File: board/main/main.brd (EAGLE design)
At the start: 108.5 x 39 mm, 40 parts, among them IC1 78m05, J1 188275-8, U1 6N138M, U2 MMBD4148TW-7-F, U3 MMBD4148TW-7-F, U4 MMBD4148TW-7-F

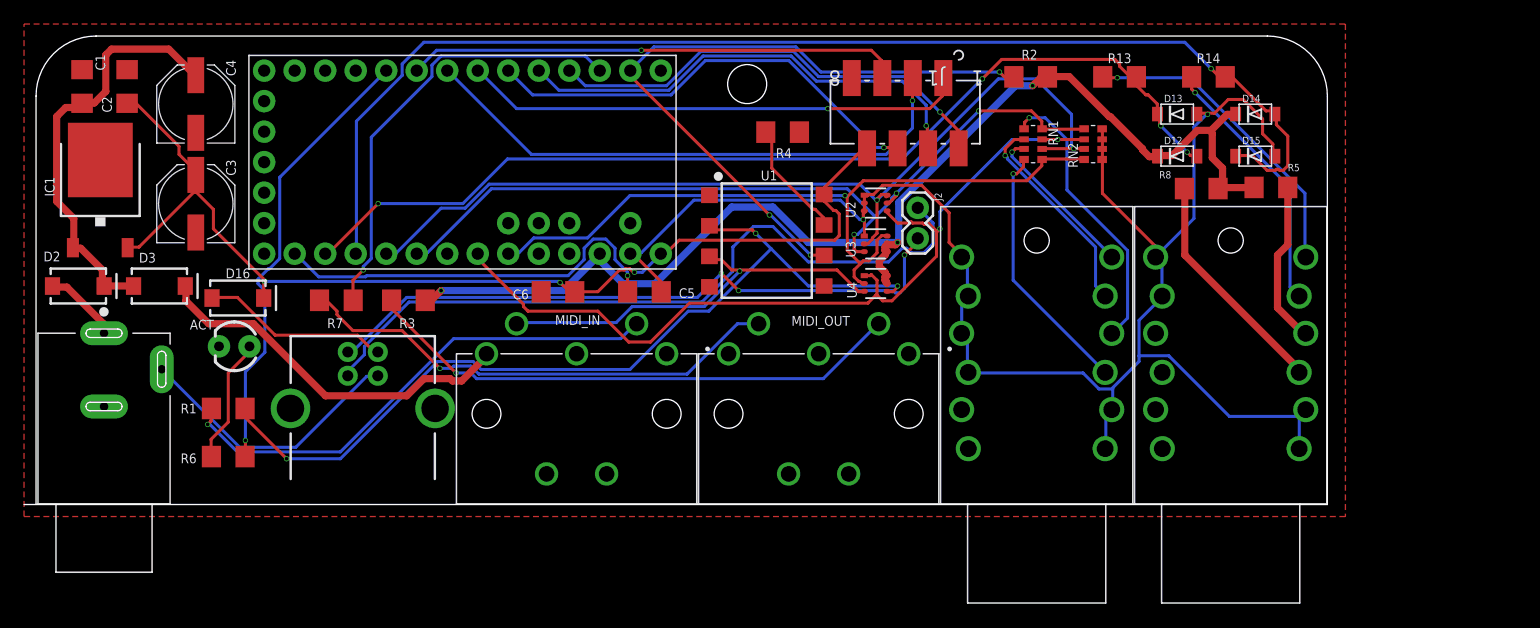
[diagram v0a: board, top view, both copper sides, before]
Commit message: Main board, revision E
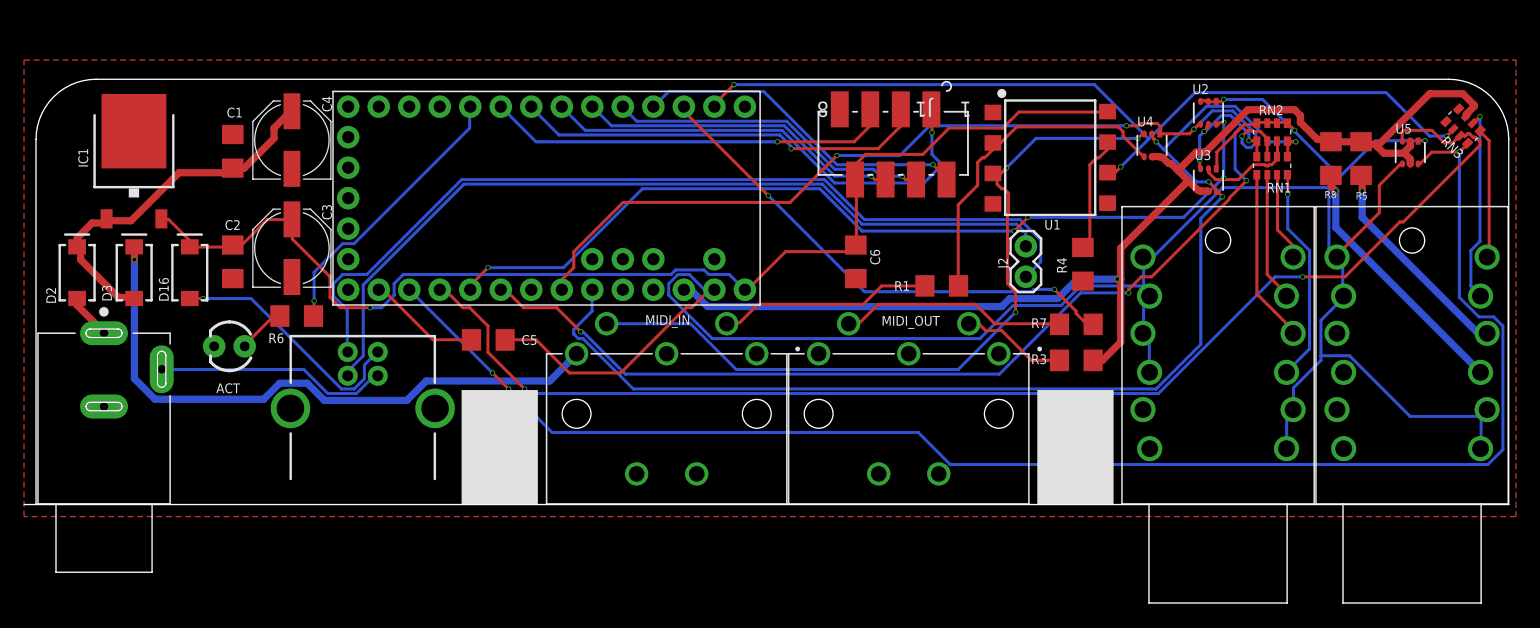
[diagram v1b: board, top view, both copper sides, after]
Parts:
- removed D12, D13, D14, D15: SM5817, adafruit:SOD-123FL
- removed R13, R14, R2: 1K, SparkFun-Resistors:1206
- added RN3: 1K, resistor-dil:EXB38V
- added U5: BAT54SDW-7-F, BAT54SDW7F:SOT-363_DIO
- moved R7 61.6 mm to (86.6, 15.0)
- moved R1 60.3 mm to (75.4, 18.2)
- moved R3 55.8 mm to (86.6, 12.0)
- moved U2 28.7 mm to (97.6, 32.6), turned to 270 degrees
- moved U3 28.2 mm to (97.6, 27.0), turned to 270 degrees
- moved R4 27.3 mm to (87.2, 20.0), turned to 270 degrees
- moved U4 25.7 mm to (92.9, 29.9), turned to 270 degrees
- moved C6 24.9 mm to (68.2, 20.2), turned to 270 degrees
- moved U1 24.6 mm to (84.6, 28.7)
- moved RN1 20.0 mm to (102.9, 28.2), turned to 0 degrees
- moved C2 17.0 mm to (16.4, 20.2), turned to 270 degrees
- moved TRIG1 15.1 mm to (98.4, 8.30)
- moved EXP 15.1 mm to (114.5, 8.30)
- moved RN2 14.9 mm to (102.9, 31.0), turned to 180 degrees
- moved C1 13.7 mm to (16.4, 29.4)
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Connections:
- net 3V: now also RN3.3, U5.2, U5.5; no longer D12.C, D14.C, R2.1
- net AGND: now also U5.1, U5.4; no longer D13.A, D15.A
- net JACK1: now also RN3.8, U5.6; no longer D12.A, D13.C, R13.2
- net JACK2: now also RN3.7, U5.3; no longer D14.A, D15.C, R14.2
- net N$18: now also RN3.1; no longer R13.1
- net N$21: now also RN3.2; no longer R14.1
- net RX: now also RN3.6; no longer R2.2
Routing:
- net AGND: track 139.8 -> 187.0 mm, vias 2 -> 3
- net JACK1: track 84.0 -> 129.4 mm, vias 4 -> 3
- net SIG-C: track 72.6 -> 27.6 mm, vias 3 -> 0
- net N$6: track 45.5 -> 8.81 mm, vias 1 -> 0
- net JACK6: track 63.9 -> 97.3 mm, vias 1 -> 4
- net SIG-A: track 34.7 -> 64.2 mm, vias 1 -> 3
- net N$3: track 42.5 -> 17.8 mm, vias 1 -> 0
- net N$4: track 33.7 -> 9.46 mm, vias 1 -> 0
- net N$8: track 41.2 -> 18.9 mm, vias 1 -> 0
- net N$5: track 31.3 -> 51.3 mm, vias 0 -> 1
- net N$13: track 54.5 -> 74.3 mm, vias 3 -> 0
- net JACK4: track 69.3 -> 88.5 mm, vias 3 -> 6
- net RX: track 56.6 -> 72.3 mm
- net N$18: track 26.2 -> 10.9 mm, vias 1 -> 0
- net ACT_LED: track 37.5 -> 23.4 mm
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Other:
- board size 108.5 x 39 mm -> 123.6 x 35.4 mm
- board text added: "11/15/2020 REV: E"
- board text removed: "11/03/2020 REV: D"
